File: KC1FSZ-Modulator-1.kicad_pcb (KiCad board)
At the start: 2 copper layers, 50 x 25 mm, 28 parts, among them J1 Conn_01x02, J2 Conn_01x02, J3 Conn_01x02, J4 Conn_01x03, J5 Conn_01x02, J6 Conn_01x02, U1 MAX4466EXK, U2 PAT1220-C-6DB, U3 BGA2867

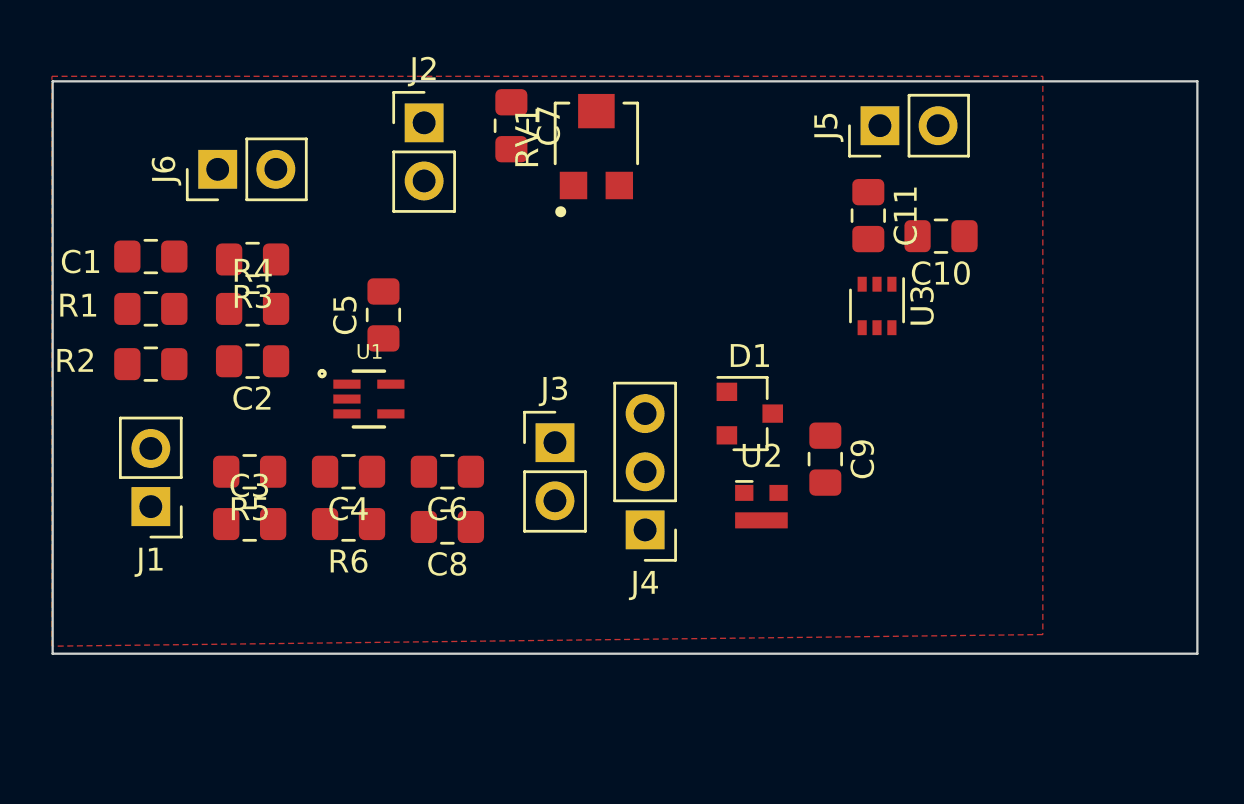
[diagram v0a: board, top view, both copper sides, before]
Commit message: Working
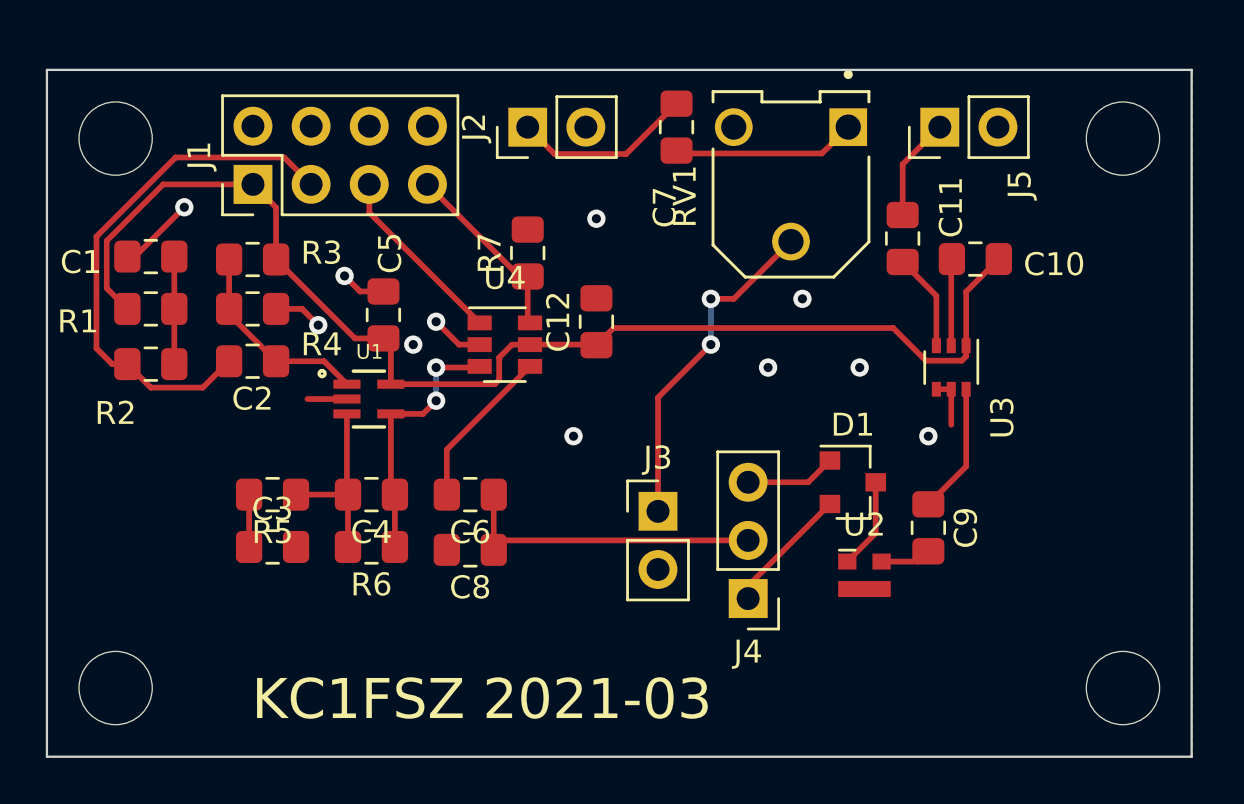
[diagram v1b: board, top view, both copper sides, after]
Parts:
- removed J6: Conn_01x02, Connector_PinHeader_2.54mm:PinHeader_1x02_P2.54mm_Vertical
- added C12: 0.1U, Capacitor_SMD:C_0805_2012Metric_Pad1.15x1.40mm_HandSolder, F.Cu at (133.0, 92.0)
- added H1: MountingHole, MountingHole:MountingHole_3.2mm_M3_ISO14580, F.Cu at (112.0, 84.0)
- added H2: MountingHole, MountingHole:MountingHole_3.2mm_M3_ISO14580, F.Cu at (156.0, 84.0)
- added H3: MountingHole, MountingHole:MountingHole_3.2mm_M3_ISO14580, F.Cu at (156.0, 108.0)
- added H4: MountingHole, MountingHole:MountingHole_3.2mm_M3_ISO14580, F.Cu at (112.0, 108.0)
- added R7: R, Resistor_SMD:R_0805_2012Metric_Pad1.15x1.40mm_HandSolder, F.Cu at (130.0, 89.0)
- added U4: TS5A3159ADBVR, Package_TO_SOT_SMD:SOT-23-6, F.Cu at (129.0, 93.0)
- J1: value Conn_01x02 -> Conn_02x04_Odd_Even; footprint Connector_PinHeader_2.54mm:PinHeader_1x02_P2.54mm_Vertical -> Connector_PinHeader_2.54mm:PinHeader_2x04_P2.54mm_Vertical
- RV1: value R_POT -> 100 (3362W); footprint TRIM_TC33X-2-104E:TRIM_TC33X-2-104E -> 3306F-1-101:TRIM_3306F-1-101
- moved J1 14.8 mm to (118.0, 86.0), turned to 90 degrees
- moved RV1 8.68 mm to (141.5, 86.0)
- moved C7 7.21 mm to (136.5, 83.5)
- moved C9 5.41 mm to (147.5, 101.0)
- moved D1 5.41 mm to (144.2, 99.0)
- moved J3 5.41 mm to (135.7, 100.3)
- moved J4 5.41 mm to (139.6, 104.1)
- moved U2 5.41 mm to (144.7, 103.1)
- moved J2 4.53 mm to (130.0, 83.5), turned to 90 degrees
- moved U3 4.21 mm to (148.5, 94.0)
- moved J5 2.62 mm to (148.0, 83.5)
- moved C10 1.80 mm to (149.6, 89.3)
- moved C11 1.80 mm to (146.4, 88.4)
- moved C3 1.41 mm to (118.9, 101.8)
- moved C4 1.41 mm to (123.2, 99.6)
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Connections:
- net Net-(C11-Pad1) renamed IF_OUT
- net Net-(C7-Pad1) renamed BFO_IN
- C2 pad 2: Net-(C2-Pad2) -> MIC_IN
- C6 pad 2: Net-(C4-Pad1) -> Net-(C6-Pad2)
- J1 pad 1: GNDA -> +5VA
- J1 pad 2: Net-(C2-Pad2) -> GNDA
- R2 pad 2: Net-(C2-Pad2) -> MIC_IN
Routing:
- net +5VA: track 0.00 -> 54.9 mm
- net MIC_IN: track 0.00 -> 23.2 mm
- net GNDA: track 0.00 -> 17.5 mm, vias 0 -> 11
- net Net-(J3-Pad1): track 0.00 -> 14.8 mm, vias 0 -> 2
- net Net-(C6-Pad1): track 0.00 -> 13.7 mm
- net Net-(C4-Pad1): track 0.00 -> 11.5 mm, vias 0 -> 2
- net Net-(C2-Pad1): track 0.00 -> 8.80 mm
- net AUDIO_SEL: track 0.00 -> 8.11 mm
- net Net-(C4-Pad2): track 0.00 -> 8.10 mm
- net LINE_IN: track 0.00 -> 8.05 mm
- net Net-(C7-Pad2): track 0.00 -> 8.03 mm
- net BFO_IN: track 0.00 -> 7.90 mm
- net Net-(C6-Pad2): track 0.00 -> 7.11 mm
- net Net-(C9-Pad1): track 0.00 -> 5.84 mm
- net Net-(D1-Pad2): track 0.00 -> 5.61 mm
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- added copper zone on B.Cu, net GNDA
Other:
- board size 50 x 25 mm -> 50 x 30 mm
- board text added: "KC1FSZ 2021-03"
